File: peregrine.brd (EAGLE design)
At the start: 55.9 x 71.1 mm, 74 parts, among them IC2 LMV358IDGKR, J1 USB MICRO, U1 ITG-3200, U2 ADXL345, U4 3.3V, U5 ATMEGA32U4-XUAU, Y1 16MHz KX-7

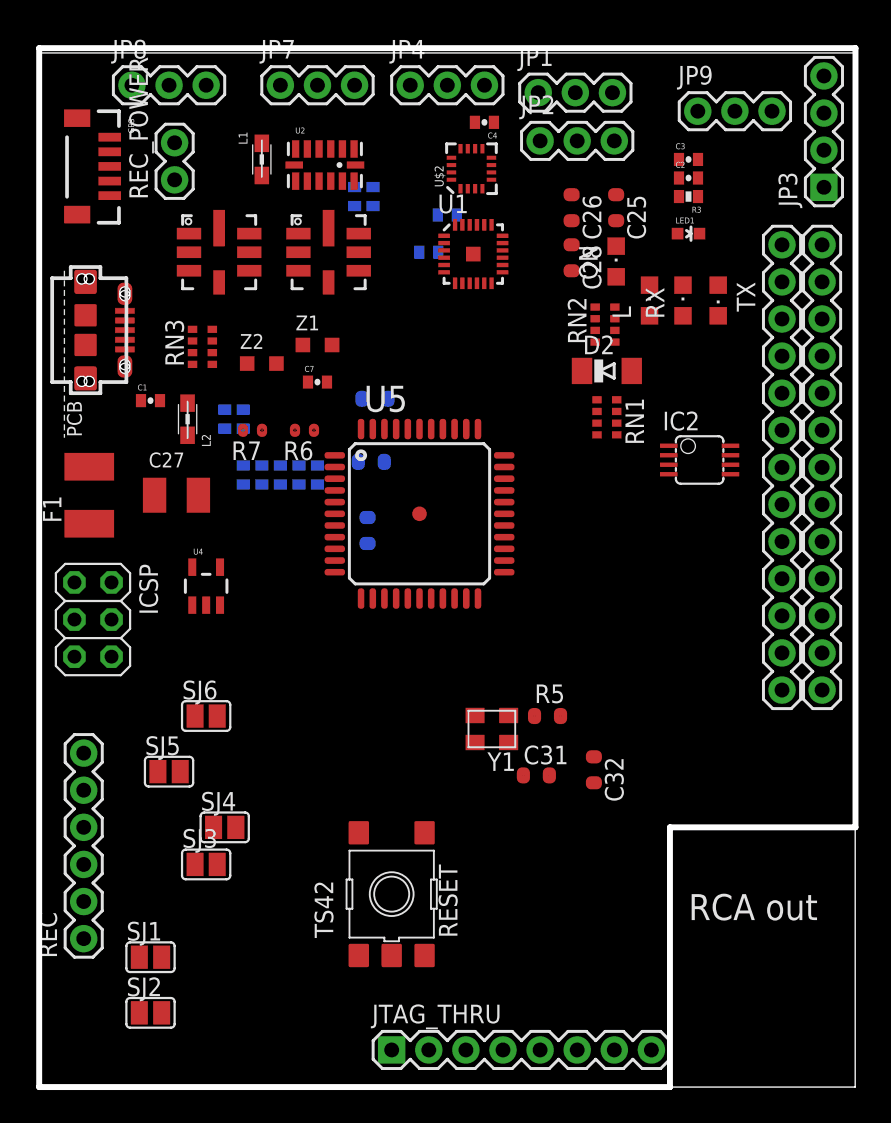
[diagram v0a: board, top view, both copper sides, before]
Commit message: Tweaked placement
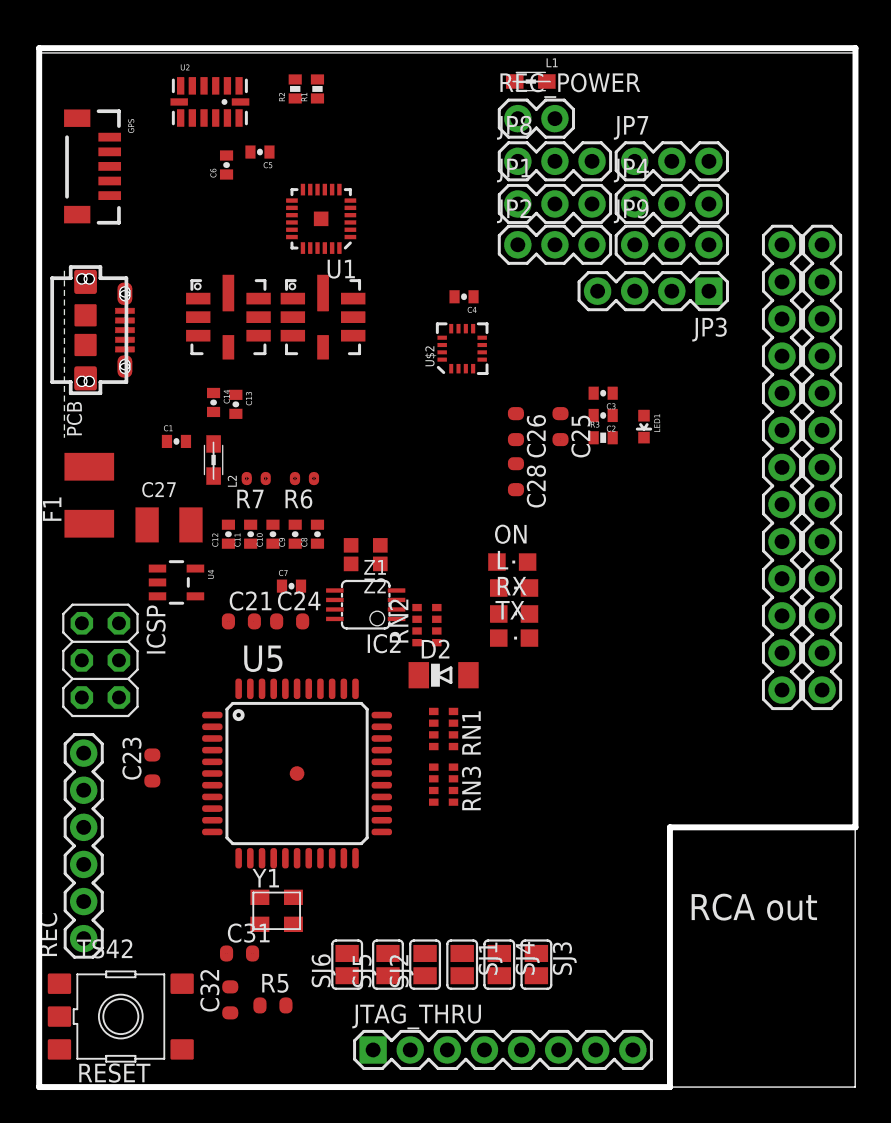
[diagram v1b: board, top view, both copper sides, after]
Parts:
- moved RN3 34.2 mm to (31.5, 24.5), turned to 90 degrees
- moved C32 29.5 mm to (16.9, 9.78), turned to 90 degrees
- moved R5 27.3 mm to (19.8, 9.40)
- moved TX 27.0 mm to (36.3, 34.5), turned to 270 degrees
- moved JP8 26.9 mm to (36.6, 67.2)
- moved IC2 24.9 mm to (26.2, 36.8), turned to 90 degrees
- moved JP7 24.8 mm to (44.6, 67.2)
- moved RX 24.4 mm to (36.3, 36.2), turned to 270 degrees
- moved RN1 24.1 mm to (31.5, 28.3)
- moved RN2 23.9 mm to (30.4, 35.4)
- moved REC_POWER 23.9 mm to (36.6, 70.1), turned to 0 degrees
- moved C31 23.7 mm to (17.5, 13.0)
- moved D2 23.6 mm to (31.5, 32.0)
- moved SJ3 23.6 mm to (37.8, 12.2), turned to 270 degrees
- moved C23 21.9 mm to (11.6, 25.7), flipped to the top, turned to 90 degrees
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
